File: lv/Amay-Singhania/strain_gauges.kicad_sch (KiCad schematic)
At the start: 21 parts, among them U2 AD8222HACPZ-R7, U3 AD8222HACPZ-R7, U6 AD8222HACPZ-R7

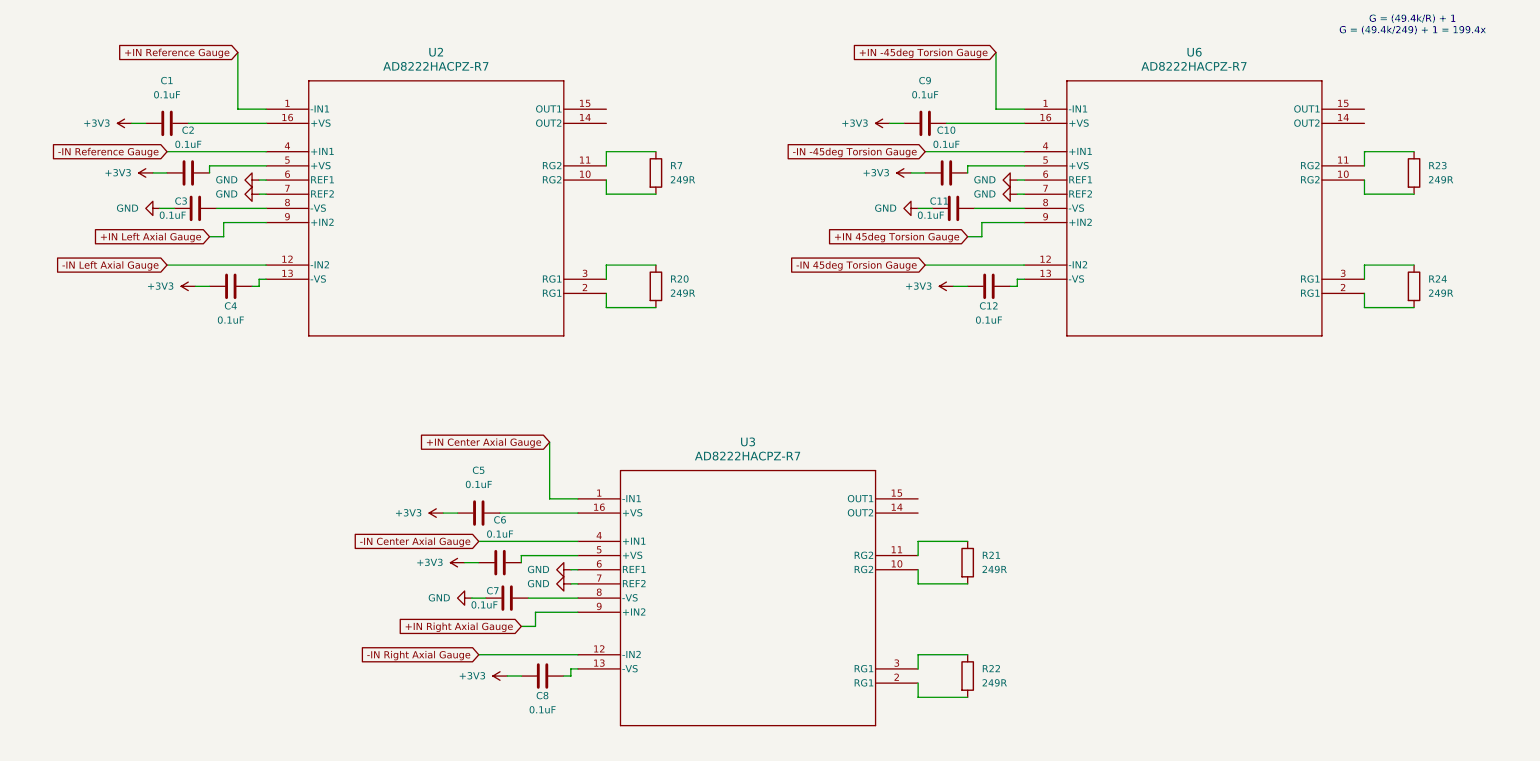
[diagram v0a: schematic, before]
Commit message: lv and fw changes
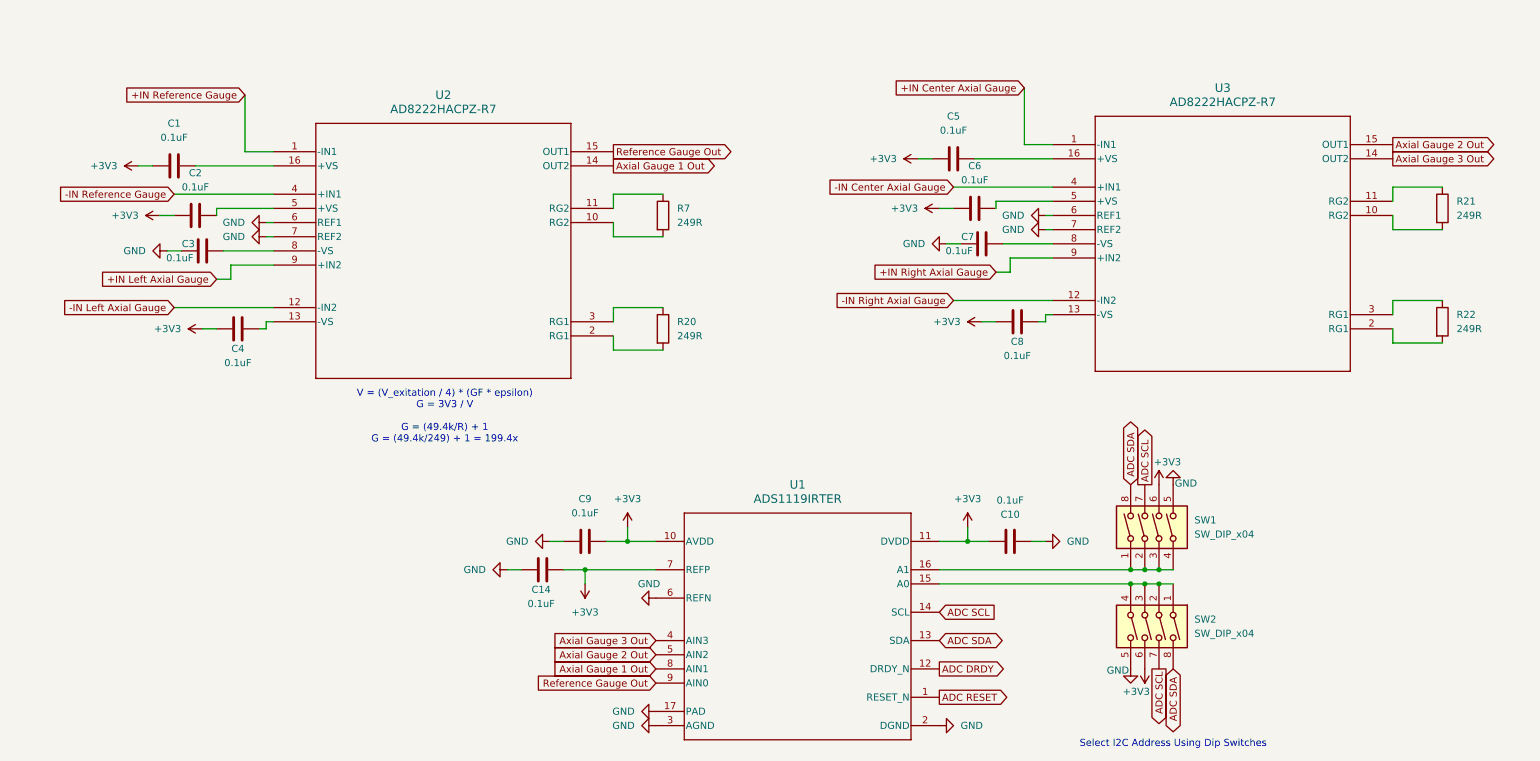
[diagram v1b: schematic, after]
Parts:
- removed C11, C12: 0.1uF, Package_TO_SOT_SMD:TSOT-23-5, symbol Device:C
- removed R23, R24: 249R, Package_DIP:DIP-8_W7.62mm, symbol Device:R
- removed U6: AD8222HACPZ-R7, AD8222:CP_16_19_ADI, symbol AD8222:AD8222HACPZ-R7
- added C14: 0.1uF, Package_TO_SOT_SMD:TSOT-23-5, symbol Device:C
- added SW1, SW2: SW_DIP_x04, RTE0016D, symbol Switch:SW_DIP_x04
- added U1: ADS1119IRTER, RTE0016D, symbol ADS1119IRTER:ADS1119IRTER
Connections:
- net +3V3: now also C14.1, SW1.6, SW2.6, U1.10 (AVDD), U1.11 (DVDD), U1.7 (REFP)
- net GND: now also C10.2, C9.2, C14.2, SW1.5, SW2.5, U1.17 (PAD), U1.2 (DGND), U1.3 (AGND), U1.6 (REFN)
- net Axial Gauge 1 Out: now reaches U2.14 (OUT2)
- net Axial Gauge 1 Out: now also U1.8 (AIN1)
- net Reference Gauge Out: now reaches U2.15 (OUT1)
- net Reference Gauge Out: now also U1.9 (AIN0)
- net Axial Gauge 3 Out: now reaches U3.14 (OUT2)
- net Axial Gauge 3 Out: now also U1.4 (AIN3)
- net Axial Gauge 2 Out: now reaches U3.15 (OUT1)
- net Axial Gauge 2 Out: now also U1.5 (AIN2)
- new net: SW2.1, SW2.2, SW2.3, SW2.4, U1.15 (A0)
- new net: SW1.1, SW1.2, SW1.3, SW1.4, U1.16 (A1)
- new net ADC DRDY: U1.12 (DRDY_N)
- new net ADC RESET: U1.1 (RESET_N)
- new net ADC SCL: SW1.7, SW2.7, U1.14 (SCL)
- new net ADC SDA: SW1.8, SW2.8, U1.13 (SDA)
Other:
- note added: "Select I2C Address Using Dip Switches"
- note added: "V = (V_exitation / 4) * (GF * epsilon) G = 3V3 / V G = (49.4k/R) + 1 G = (49.4k/249) + 1 = 199.4x"
- note removed: "G = (49.4k/R) + 1 G = (49.4k/249) + 1 = 199.4x"
- moved on the sheet: C1, C2, C3, C4, C5, C6, C7, C8, R20, R21, R22, R7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
